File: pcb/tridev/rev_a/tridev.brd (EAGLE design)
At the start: 108 x 72.4 mm, 66 parts, among them J1 MICRO_USB_B_HIROSE_ZX62R-B-5P, J5 TC2030-JLINK-L, J6 TC2030-JLINK-L, U1 TRIPOINT-BREAKOUT, U2 NRF51822QF, U3 MAX8887EZK33+T, U4 FT232HQ, X1 EPSON-FA-128, X2 TXC-8Z-12MHZ

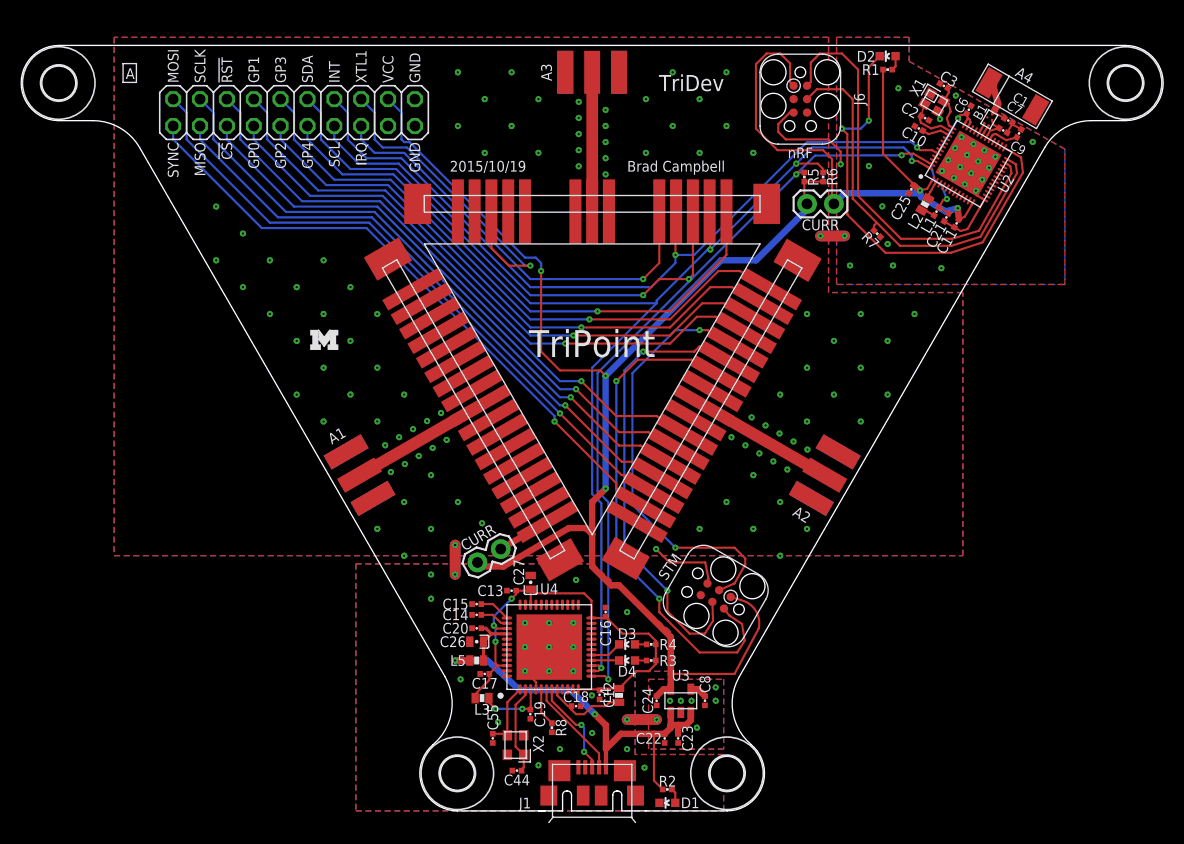
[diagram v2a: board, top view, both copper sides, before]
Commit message: revert tridev to version that was fabbed
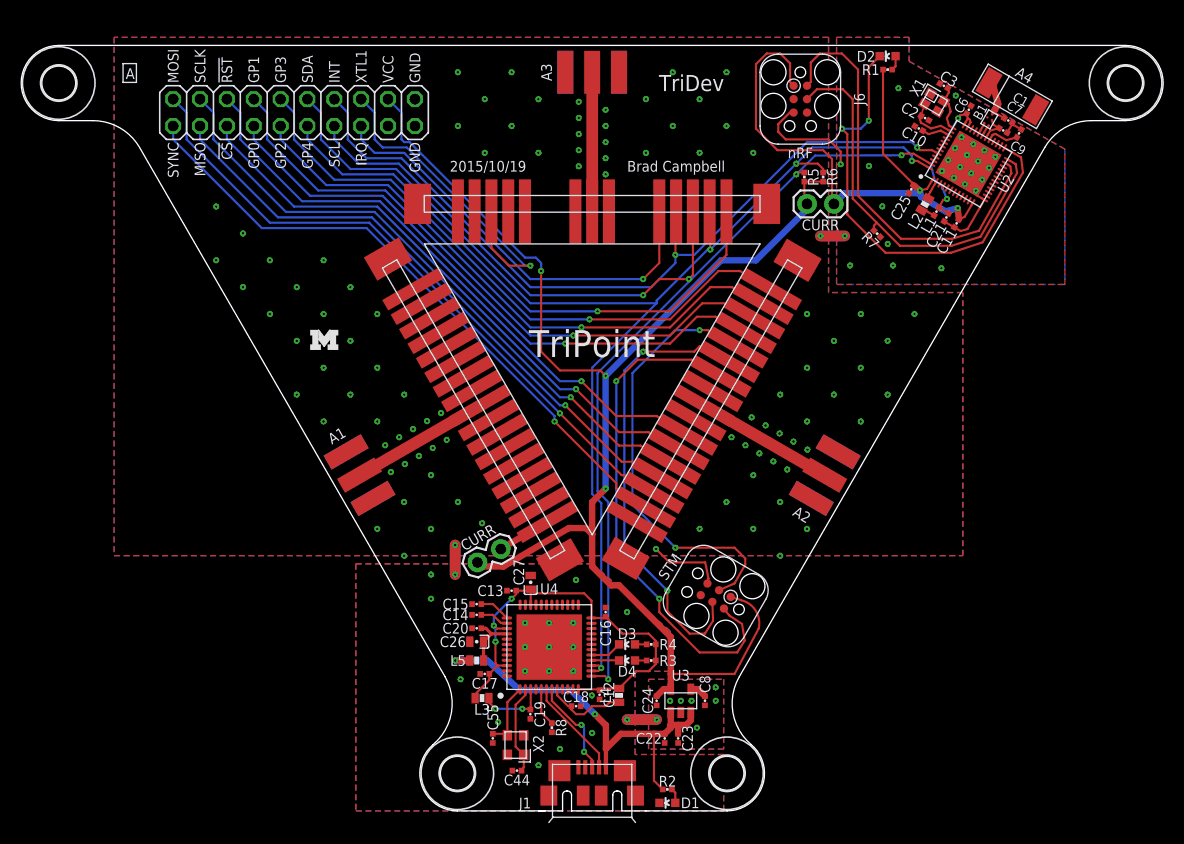
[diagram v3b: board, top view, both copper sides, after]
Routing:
- net GND: track 44.7 -> 42.6 mm, vias 154 -> 150
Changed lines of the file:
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@@
 <grid distance="10" unitdist="mil" unit="mil" style="lines" multiple="1" display="yes" altdistance="1" altunitdist="mil" altunit="mil"/>
 <layers>
-<layer number="1" name="Top" color="4" fill="1" visible="yes" active="yes"/>
+<layer number="1" name="Top" color="4" fill="1" visible="no" active="yes"/>
 <layer number="2" name="Route2" color="1" fill="3" visible="no" active="no"/>
 <layer number="3" name="Route3" color="4" fill="3" visible="no" active="no"/>
@@
 <layer number="14" name="Route14" color="1" fill="6" visible="no" active="no"/>
 <layer number="15" name="Route15" color="4" fill="6" visible="no" active="no"/>
-<layer number="16" name="Bottom" color="1" fill="1" visible="yes" active="yes"/>
+<layer number="16" name="Bottom" color="1" fill="1" visible="no" active="yes"/>
 <layer number="17" name="Pads" color="2" fill="1" visible="yes" active="yes"/>
 <layer number="18" name="Vias" color="2" fill="1" visible="yes" active="yes"/>
 <layer number="19" name="Unrouted" color="13" fill="1" visible="yes" active="yes"/>
 <layer number="20" name="Dimension" color="15" fill="1" visible="yes" active="yes"/>
-<layer number="21" name="tPlace" color="7" fill="1" visible="yes" active="yes"/>
-<layer number="22" name="bPlace" color="7" fill="1" visible="yes" active="yes"/>
-<layer number="23" name="tOrigins" color="15" fill="1" visible="yes" active="yes"/>
-<layer number="24" name="bOrigins" color="15" fill="1" visible="yes" active="yes"/>
-<layer number="25" name="tNames" color="7" fill="1" visible="yes" active="yes"/>
-<layer number="26" name="bNames" color="7" fill="1" visible="yes" active="yes"/>
+<layer number="21" name="tPlace" color="7" fill="1" visible="no" active="yes"/>
+<layer number="22" name="bPlace" color="7" fill="1" visible="no" active="yes"/>
+<layer number="23" name="tOrigins" color="15" fill="1" visible="no" active="yes"/>
+<layer number="24" name="bOrigins" color="15" fill="1" visible="no" active="yes"/>
+<layer number="25" name="tNames" color="7" fill="1" visible="no" active="yes"/>
+<layer number="26" name="bNames" color="7" fill="1" visible="no" active="yes"/>
 <layer number="27" name="tValues" color="7" fill="1" visible="no" active="yes"/>
 <layer number="28" name="bValues" color="7" fill="1" visible="no" active="yes"/>
@@
 <layer number="37" name="tTest" color="7" fill="1" visible="no" active="yes"/>
 <layer number="38" name="bTest" color="7" fill="1" visible="no" active="yes"/>
-<layer number="39" name="tKeepout" color="4" fill="11" visible="yes" active="yes"/>
-<layer number="40" name="bKeepout" color="1" fill="11" visible="yes" active="yes"/>
-<layer number="41" name="tRestrict" color="4" fill="10" visible="yes" active="yes"/>
-<layer number="42" name="bRestrict" color="1" fill="10" visible="yes" active="yes"/>
-<layer number="43" name="vRestrict" color="2" fill="10" visible="yes" active="yes"/>
+<layer number="39" name="tKeepout" color="4" fill="11" visible="no" active="yes"/>
+<layer number="40" name="bKeepout" color="1" fill="11" visible="no" active="yes"/>
+<layer number="41" name="tRestrict" color="4" fill="10" visible="no" active="yes"/>
+<layer number="42" name="bRestrict" color="1" fill="10" visible="no" active="yes"/>
+<layer number="43" name="vRestrict" color="2" fill="10" visible="no" active="yes"/>
 <layer number="44" name="Drills" color="7" fill="1" visible="no" active="yes"/>
-<layer number="45" name="Holes" color="7" fill="1" visible="yes" active="yes"/>
+<layer number="45" name="Holes" color="7" fill="1" visible="no" active="yes"/>
 <layer number="46" name="Milling" color="3" fill="1" visible="no" active="yes"/>
 <layer number="47" name="Measures" color="7" fill="1" visible="no" active="yes"/>
@@
 <layer number="106" name="bPlate" color="7" fill="1" visible="no" active="yes"/>
 <layer number="107" name="Crop" color="7" fill="1" visible="no" active="yes"/>
-<layer number="108" name="fp8" color="7" fill="1" visible="yes" active="yes"/>
-<layer number="109" name="fp9" color="7" fill="1" visible="yes" active="yes"/>
-<layer number="110" name="fp0" color="7" fill="1" visible="yes" active="yes"/>
-<layer number="111" name="LPC17xx" color="7" fill="1" visible="yes" active="yes"/>
-<layer number="112" name="tSilk" color="7" fill="1" visible="yes" active="yes"/>
-<layer number="113" name="IDFDebug" color="4" fill="1" visible="yes" active="yes"/>
+<layer number="108" name="fp8" color="7" fill="1" visible="no" active="yes"/>
+<layer number="109" name="fp9" color="7" fill="1" visible="no" active="yes"/>
+<layer number="110" name="fp0" color="7" fill="1" visible="no" active="yes"/>
+<layer number="111" name="LPC17xx" color="7" fill="1" visible="no" active="yes"/>
+<layer number="112" name="tSilk" color="7" fill="1" visible="no" active="yes"/>
+<layer number="113" name="IDFDebug" color="4" fill="1" visible="no" active="yes"/>
 <layer number="116" name="Patch_BOT" color="9" fill="4" visible="no" active="yes"/>
 <layer number="121" name="_tsilk" color="7" fill="1" visible="no" active="yes"/>
 <layer number="122" name="_bsilk" color="7" fill="1" visible="no" active="yes"/>
-<layer number="123" name="tTestmark" color="7" fill="1" visible="yes" active="yes"/>
-<layer number="124" name="bTestmark" color="7" fill="1" visible="yes" active="yes"/>
+<layer number="123" name="tTestmark" color="7" fill="1" visible="no" active="yes"/>
+<layer number="124" name="bTestmark" color="7" fill="1" visible="no" active="yes"/>
 <layer number="125" name="_tNames" color="7" fill="1" visible="no" active="yes"/>
-<layer number="126" name="_bNames" color="7" fill="1" visible="yes" active="yes"/>
-<layer number="127" name="_tValues" color="7" fill="1" visible="yes" active="yes"/>
-<layer number="128" name="_bValues" color="7" fill="1" visible="yes" active="yes"/>
-<layer number="131" name="tAdjust" color="7" fill="1" visible="yes" active="yes"/>
-<layer number="132" name="bAdjust" color="7" fill="1" visible="yes" active="yes"/>
+<layer number="126" name="_bNames" color="7" fill="1" visible="no" active="yes"/>
+<layer number="127" name="_tValues" color="7" fill="1" visible="no" active="yes"/>
+<layer number="128" name="_bValues" color="7" fill="1" visible="no" active="yes"/>
+<layer number="131" name="tAdjust" color="7" fill="1" visible="no" active="yes"/>
+<layer number="132" name="bAdjust" color="7" fill="1" visible="no" active="yes"/>
 <layer number="144" name="Drill_legend" color="7" fill="1" visible="no" active="yes"/>
-<layer number="150" name="Notes" color="7" fill="1" visible="yes" active="yes"/>
+<layer number="150" name="Notes" color="7" fill="1" visible="no" active="yes"/>
 <layer number="151" name="HeatSink" color="7" fill="1" visible="no" active="yes"/>
-<layer number="152" name="_bDocu" color="7" fill="1" visible="yes" active="yes"/>
-<layer number="153" name="FabDoc1" color="7" fill="1" visible="yes" active="yes"/>
-<layer number="154" name="FabDoc2" color="7" fill="1" visible="yes" active="yes"/>
-<layer number="155" name="FabDoc3" color="7" fill="1" visible="yes" active="yes"/>
-<layer number="199" name="Contour" color="7" fill="1" visible="yes" active="yes"/>
-<layer number="200" name="200bmp" color="1" fill="10" visible="yes" active="yes"/>
-<layer number="201" name="201bmp" color="1" fill="10" visible="yes" active="yes"/>
-<layer number="202" name="202bmp" color="3" fill="10" visible="yes" active="yes"/>
+<layer number="152" name="_bDocu" color="7" fill="1" visible="no" active="yes"/>
+<layer number="153" name="FabDoc1" color="7" fill="1" visible="no" active="yes"/>
+<layer number="154" name="FabDoc2" color="7" fill="1" visible="no" active="yes"/>
+<layer number="155" name="FabDoc3" color="7" fill="1" visible="no" active="yes"/>
+<layer number="199" name="Contour" color="7" fill="1" visible="no" active="yes"/>
+<layer number="200" name="200bmp" color="1" fill="10" visible="no" active="yes"/>
+<layer number="201" name="201bmp" color="1" fill="10" visible="no" active="yes"/>
+<layer number="202" name="202bmp" color="3" fill="10" visible="no" active="yes"/>
 <layer number="203" name="203bmp" color="4" fill="10" visible="no" active="yes"/>
 <layer number="204" name="204bmp" color="5" fill="10" visible="no" active="yes"/>
@@
 <layer number="223" name="223bmp" color="24" fill="1" visible="no" active="no"/>
 <layer number="224" name="224bmp" color="25" fill="1" visible="no" active="no"/>
-<layer number="248" name="Housing" color="7" fill="1" visible="yes" active="yes"/>
-<layer number="249" name="Edge" color="7" fill="1" visible="yes" active="yes"/>
+<layer number="248" name="Housing" color="7" fill="1" visible="no" active="yes"/>
+<layer number="249" name="Edge" color="7" fill="1" visible="no" active="yes"/>
 <layer number="250" name="Descript" color="3" fill="1" visible="no" active="no"/>
 <layer number="251" name="SMDround" color="12" fill="11" visible="no" active="no"/>
@@
 <via x="-17.719590625" y="-11.64996875" extent="1-16" drill="0.2032"/>
 <via x="-19.039415625" y="-12.41196875" extent="1-16" drill="0.2032"/>
-<via x="41.660090625" y="18.813975" extent="1-16" drill="0.2032"/>
-<via x="32.897090625" y="20.972975" extent="1-16" drill="0.2032"/>
-<via x="3.302" y="-38.608" extent="1-16" drill="0.2032"/>
-<via x="4.953" y="-40.3606" extent="1-16" drill="0.2032"/>
-<wire x1="-5.314" y1="-32.956" x2="-5.314" y2="-32.278" width="0.2032" layer="1"/>
-<wire x1="-5.314" y1="-32.278" x2="-6.35" y2="-31.242" width="0.2032" layer="1"/>
+<wire x1="-6.35" y1="-31.242" x2="-5.314" y2="-32.956" width="0" layer="19" extent="1-1"/>
+<wire x1="31.855815625" y1="20.851925" x2="30.511003125" y2="20.308375" width="0" layer="19" extent="1-1"/>
+<wire x1="39.247190625" y1="19.683540625" x2="37.37505" y2="21.133665625" width="0" layer="19" extent="1-1"/>
+<wire x1="6.362" y1="-43.688" x2="6.858" y2="-38.02506875" width="0" layer="19" extent="1-1"/>
 </signal>
 <signal name="VCC">
